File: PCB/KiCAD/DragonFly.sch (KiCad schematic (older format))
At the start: 31 parts, among them Q1 MMBFJ310LT1G, Q2 MMBT2222A, T2 1_4, U1 ADE-1, Y1 8Mhz, Y2 8Mhz, Y3 8Mhz, Y4 8Mhz, Y5 8Mhz, Y6 8Mhz

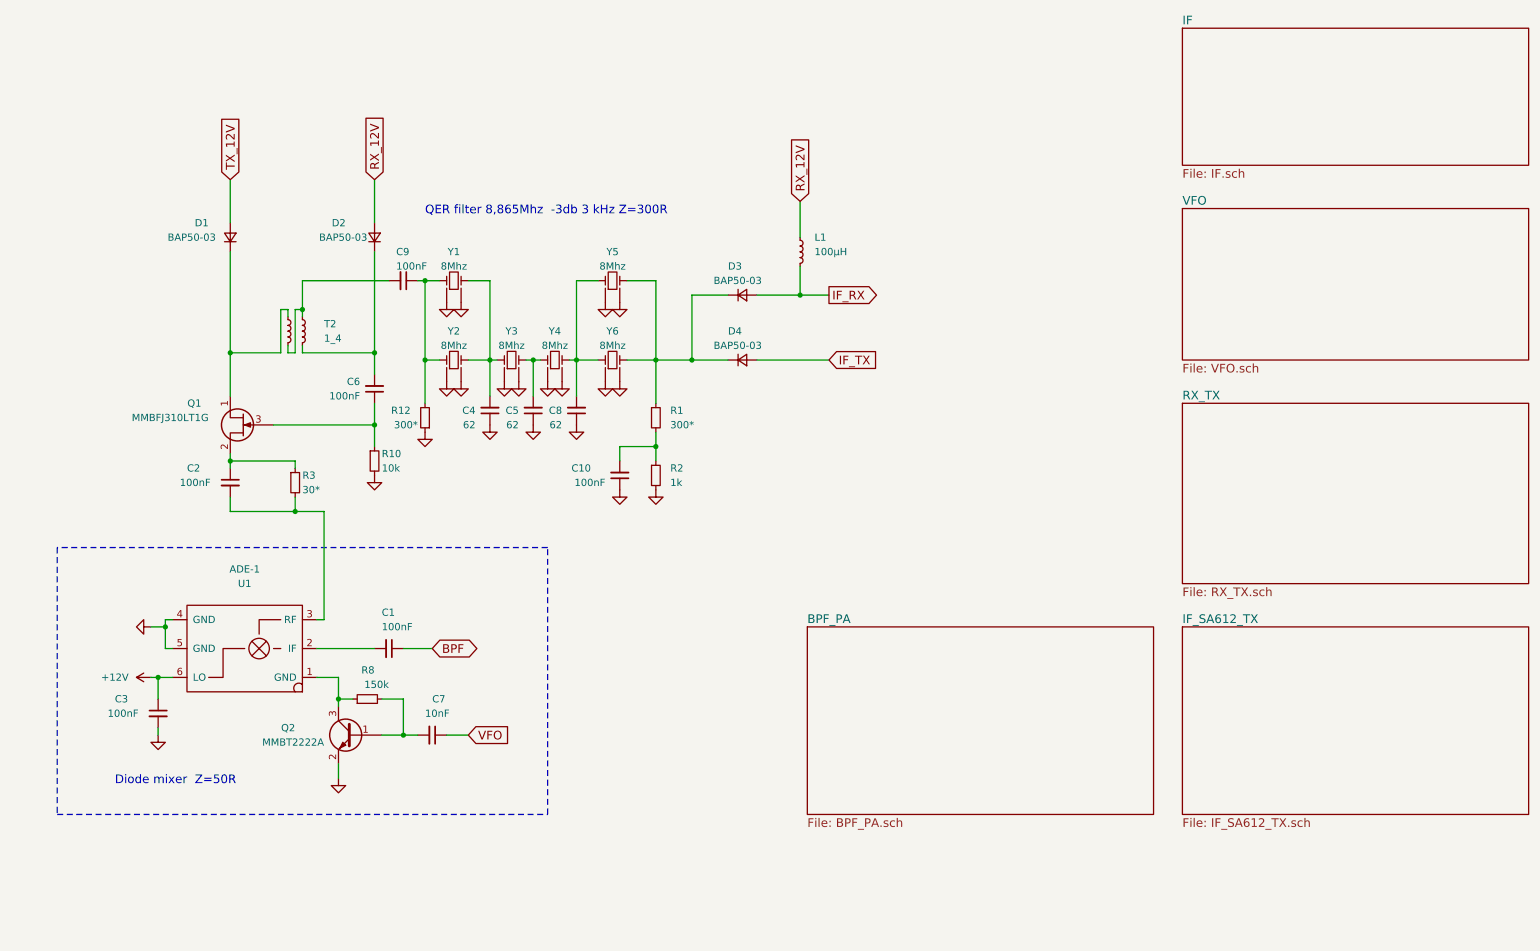
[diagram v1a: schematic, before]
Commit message: PCB home
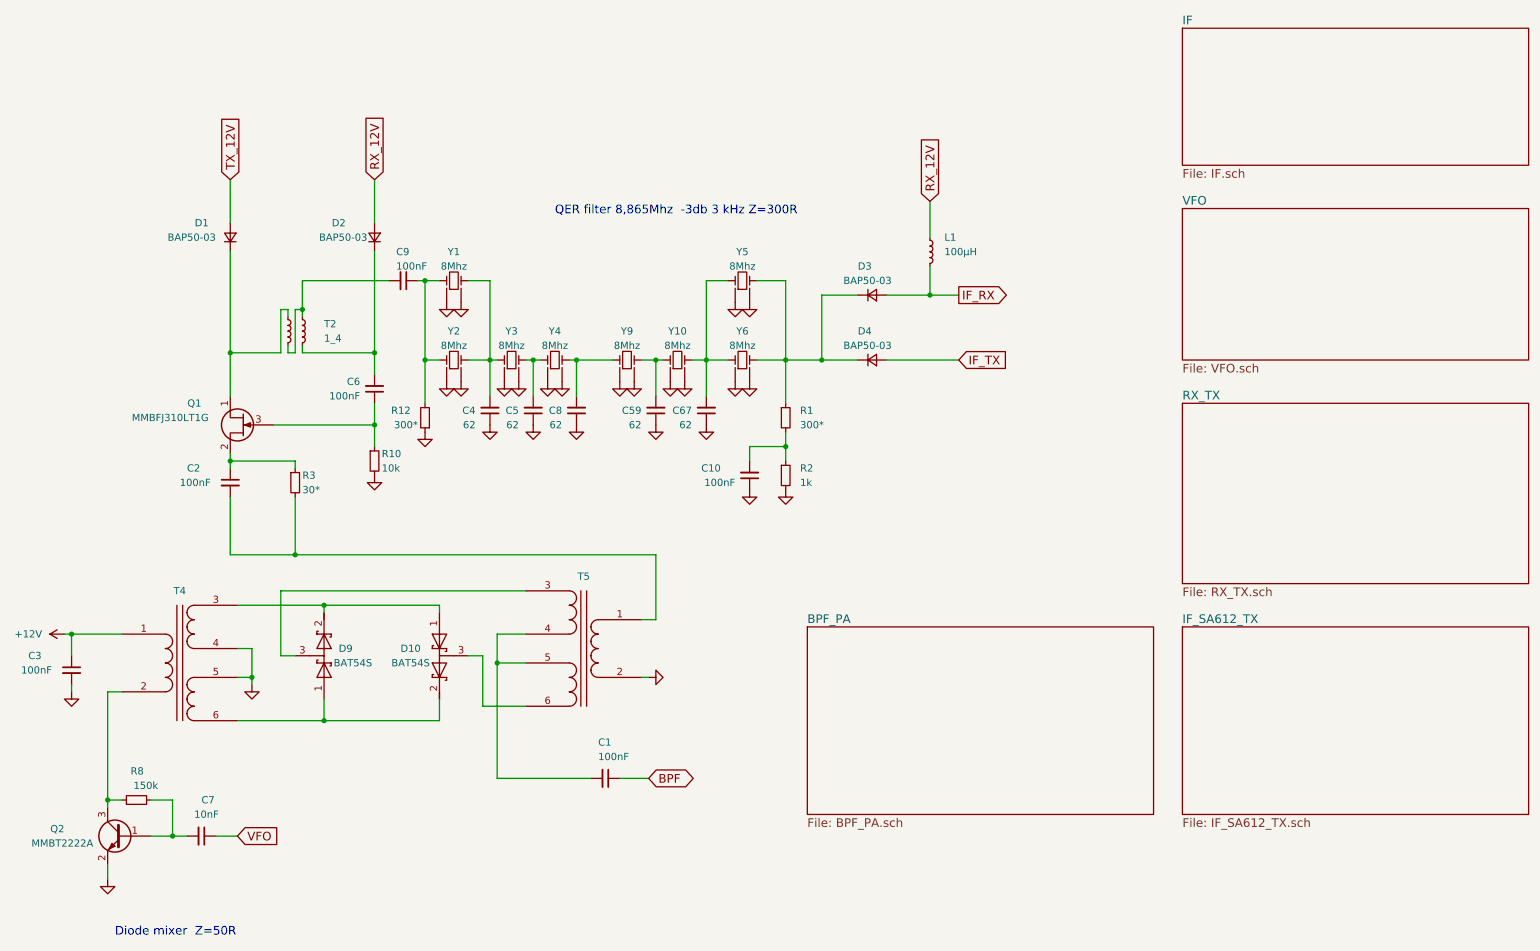
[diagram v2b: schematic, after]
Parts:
- removed U1: ADE-1, DragonFly:ADE-1H, symbol ADE-1
- added C59, C67: 62, Capacitors_SMD:C_0805, symbol C_Small
- added D10, D9: BAT54S, TO_SOT_Packages_SMD:SOT-23, symbol D_Schottky_x2_Serial_AKC
- added T4, T5: Transformer_1P_2S, DragonFly:HF12, symbol Transformer_1P_2S
- added Y10, Y9: 8Mhz, DragonFly:Crystal_HC49-U_Vertical, symbol Crystal_Filter
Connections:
- net +12V: now also T4.1 (AA)
- net GND: now also C59.1, C67.1, T4.4 (SB), T4.5 (SC), T5.2 (AB), Y10.3 (GND), Y10.4 (GND), Y9.3 (GND), Y9.4 (GND)
- net at Q2.3 (C), R8.1: now also T4.2 (AB)
- net at Y5.1, Y6.1: now also C67.2, Y10.2; no longer C8.2, Y4.2
- net at C2.2, R3.2: now also T5.1 (AA)
- net at C1.2: now also T5.4 (SB), T5.5 (SC)
- new net: C8.2, Y4.2, Y9.1
- new net: D9.3 (common), T5.3 (SA)
- new net: D10.3 (common), T5.6 (SD)
- new net: D10.1 (A), D9.2 (K), T4.3 (SA)
- new net: D10.2 (K), D9.1 (A), T4.6 (SD)
- new net: C59.2, Y10.1, Y9.2
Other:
- moved on the sheet: C1, C10, C3, C7, D3, D4, L1, Q2, R1, R2, R8, Y5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
